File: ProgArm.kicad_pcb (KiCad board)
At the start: 2 copper layers, 40 x 70 mm, 103 parts, among them J1 MICROSD_SOCKET_SPI, M1 MOTOR, P1 I2C_Port, P2 I2C_Solder, P3 SPI_Port, P4 SPI_Solder, P5 JTAG_Interface, P6 Unused_Pins, P7 HC-05/06, P8 Ring_Port, P9 MicroUSB, Q1 MOS_P, Q10 MOS_P, Q11 MOS_P, Q12 MOS_P, Q2 MOS_N, Q3 MOS_N, Q4 MOS_P, Q5 MOS_P, Q6 MOS_P, Q7 MOS_P, Q8 MOS_P, Q9 MOS_P, SW1 ON/OFF, SW2 SWITCH_INV, U1 STM32F103R, U2 LTC2942-1, U3 BMP085, U4 HMC5883L, U5 MPU6050, X1 32.768(MS3V-T1R), X2 8 mHz

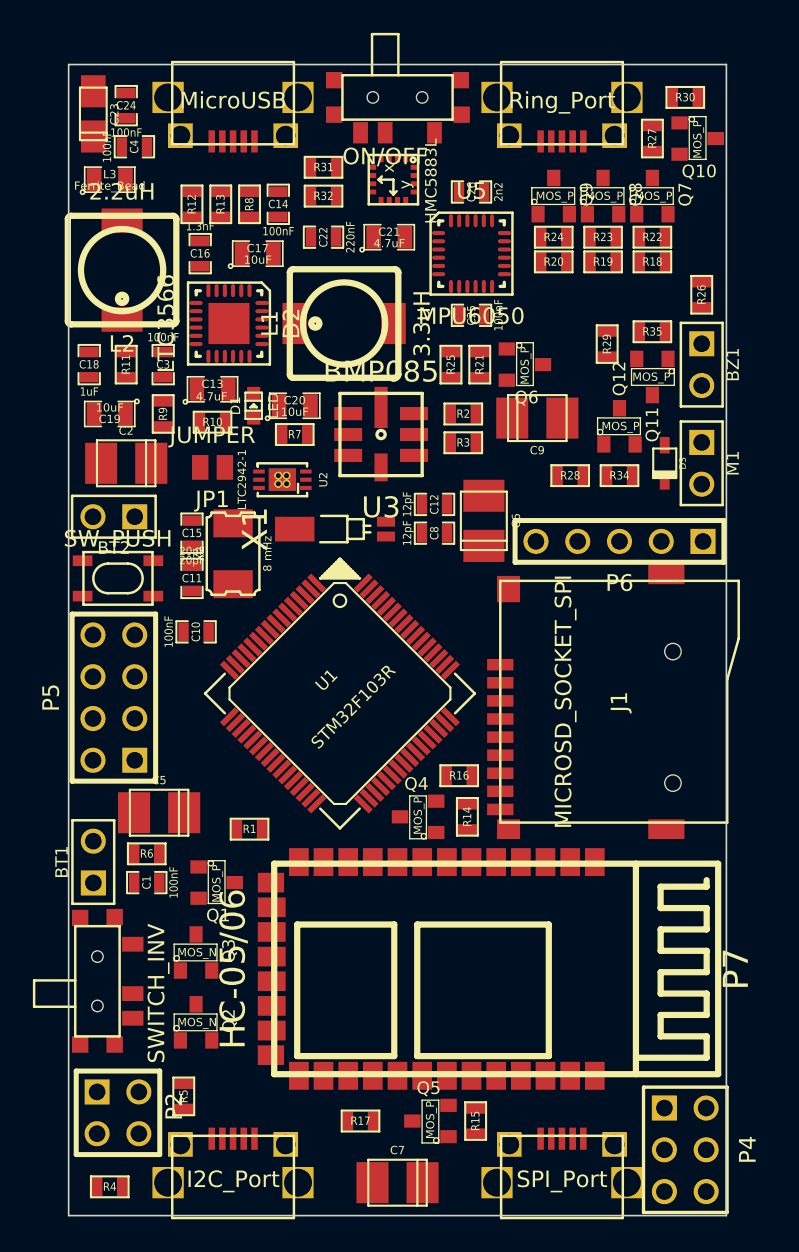
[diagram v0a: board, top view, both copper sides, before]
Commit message: ---
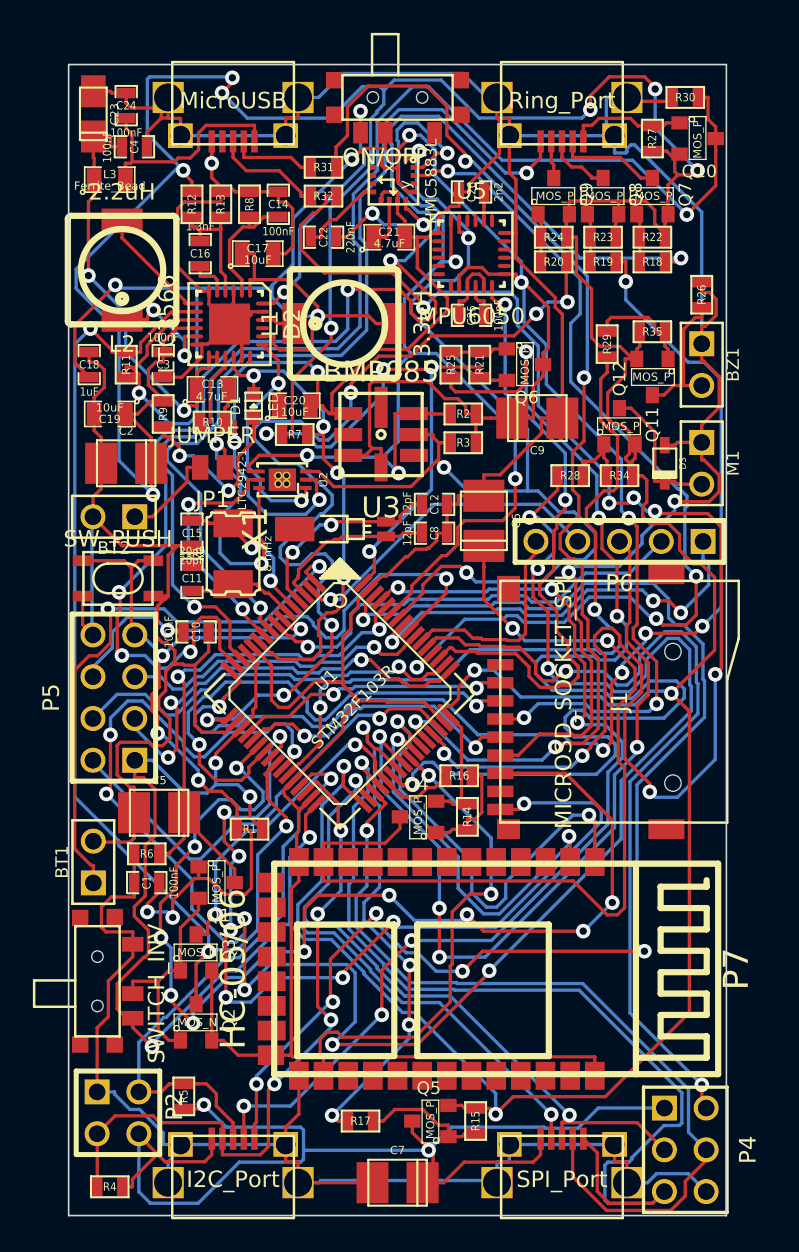
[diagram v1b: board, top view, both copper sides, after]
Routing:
- net GND: track 0.00 -> 457.3 mm, vias 0 -> 6
- net +3.3V: track 0.00 -> 351.8 mm, vias 0 -> 19
- net ~VIBRATION: track 0.00 -> 114.5 mm, vias 0 -> 10
- net D+: track 0.00 -> 93.3 mm, vias 0 -> 8
- net SYS_POWER: track 0.00 -> 92.3 mm, vias 0 -> 5
- net /~LED_R: track 0.00 -> 89.7 mm, vias 0 -> 6
- net /I2C_EXTRA2: track 0.00 -> 82.1 mm, vias 0 -> 6
- net RING_BTN1: track 0.00 -> 77.1 mm, vias 0 -> 2
- net SDA: track 0.00 -> 75.0 mm, vias 0 -> 5
- net ~SYS_PWR_ENABLE: track 0.00 -> 74.1 mm, vias 0 -> 4
- net Vout: track 0.00 -> 72.9 mm, vias 0 -> 4
- net /~LED_G: track 0.00 -> 71.0 mm, vias 0 -> 6
- net PORT_POWER: track 0.00 -> 70.5 mm, vias 0 -> 2
- net SCL: track 0.00 -> 70.0 mm, vias 0 -> 4
- net /SD_MISO: track 0.00 -> 69.3 mm, vias 0 -> 10
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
